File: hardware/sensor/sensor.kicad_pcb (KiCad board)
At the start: 2 copper layers, 83.8 x 68.6 mm, 10 parts

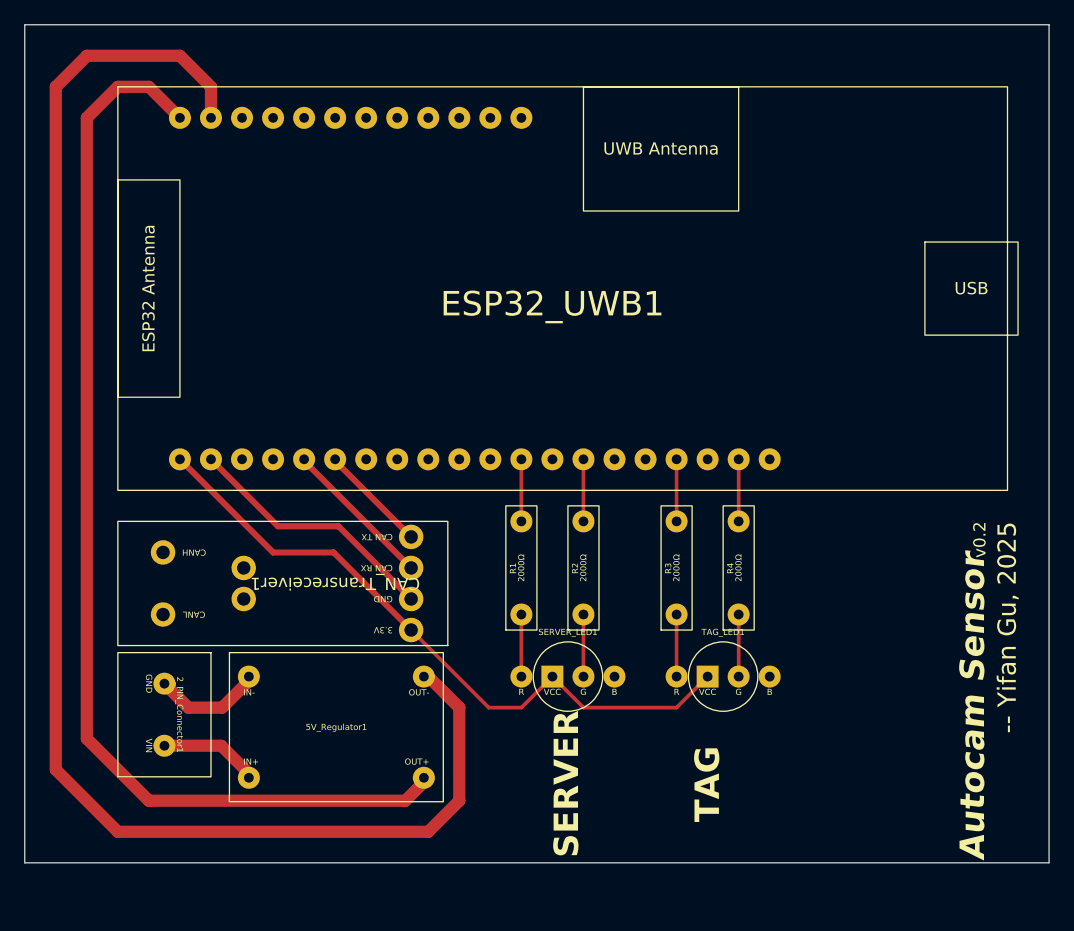
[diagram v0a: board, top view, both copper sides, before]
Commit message: hardware: Add remote PCB.
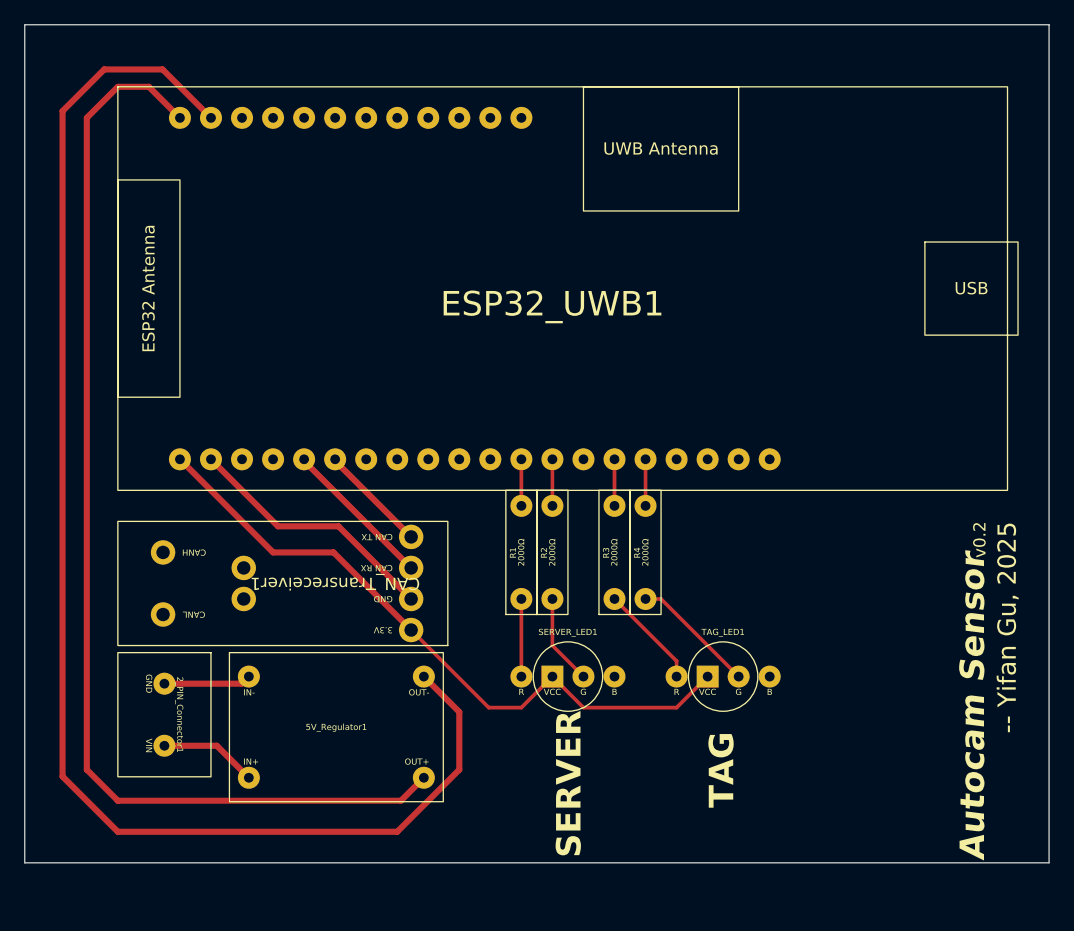
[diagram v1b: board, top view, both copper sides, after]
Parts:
- SERVER_LED1: value ~ -> SERVER
- TAG_LED1: value ~ -> TAG
- moved R4 7.73 mm to (170.2, 110.5)
- moved R3 5.24 mm to (167.6, 110.5)
- moved R2 2.84 mm to (162.6, 110.5)
- moved R1 1.27 mm to (160.0, 110.5)
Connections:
- ESP32_UWB1 pad 13: unconnected-(ESP32_UWB1-IO26-Pad13) -> Net-(ESP32_UWB1-IO26)
- ESP32_UWB1 pad 14: Net-(ESP32_UWB1-IO27) -> unconnected-(ESP32_UWB1-IO27-Pad14)
- ESP32_UWB1 pad 15: unconnected-(ESP32_UWB1-IO32-Pad15) -> Net-(ESP32_UWB1-IO32)
- ESP32_UWB1 pad 16: unconnected-(ESP32_UWB1-IO33-Pad16) -> Net-(ESP32_UWB1-IO33)
- ESP32_UWB1 pad 17: Net-(ESP32_UWB1-IO34) -> unconnected-(ESP32_UWB1-IO34-Pad17)
- ESP32_UWB1 pad 19: Net-(ESP32_UWB1-IO36) -> unconnected-(ESP32_UWB1-IO36-Pad19)
- R2 pad 2: Net-(ESP32_UWB1-IO27) -> Net-(ESP32_UWB1-IO26)
- R3 pad 2: Net-(ESP32_UWB1-IO34) -> Net-(ESP32_UWB1-IO32)
- R4 pad 2: Net-(ESP32_UWB1-IO36) -> Net-(ESP32_UWB1-IO33)
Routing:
- net Net-(5V_Regulator1-OUT-): track 120.6 -> 114.9 mm
- net Net-(TAG_LED1-G): track 5.08 -> 10.3 mm
- net Net-(ESP32_UWB1-IO36): track 5.08 -> 0.00 mm
- net Net-(ESP32_UWB1-IO34): track 5.08 -> 0.00 mm
- net Net-(ESP32_UWB1-IO27): track 5.08 -> 0.00 mm
- net Net-(ESP32_UWB1-IO33): track 0.00 -> 3.81 mm
- net Net-(ESP32_UWB1-IO32): track 0.00 -> 3.81 mm
- net Net-(ESP32_UWB1-IO26): track 0.00 -> 3.81 mm
- net Net-(TAG_LED1-R): track 5.08 -> 8.45 mm
- net Net-(SERVER_LED1-G): track 5.08 -> 7.40 mm
- net Net-(2_PIN_Connector1-Pin_1): track 9.13 -> 7.15 mm
- net Net-(SERVER_LED1-R): track 5.08 -> 6.35 mm
- net Net-(ESP32_UWB1-IO25): track 5.08 -> 3.81 mm
- net Net-(5V_Regulator1-OUT+): track 91.3 -> 92.5 mm
